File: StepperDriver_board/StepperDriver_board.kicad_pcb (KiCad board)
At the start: 2 copper layers, 50 x 70 mm, 18 parts, among them J1 Conn_01x02, J2 Conn_01x02, J3 Conn_01x02, J4 Conn_01x04_Male, J5 Conn_01x02, J6 Conn_01x04_Male, J7 Conn_01x02, J9 Conn_01x04_Male

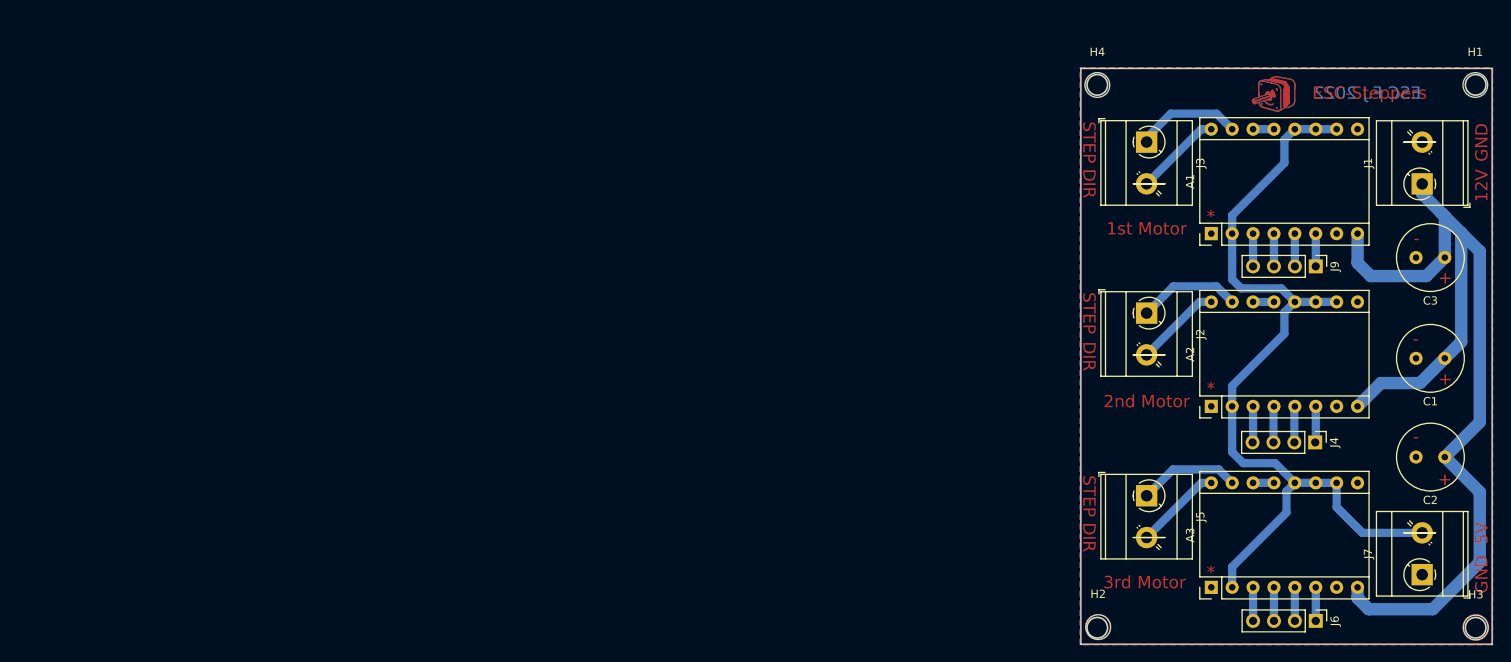
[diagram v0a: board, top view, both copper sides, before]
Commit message: Feat: add assets
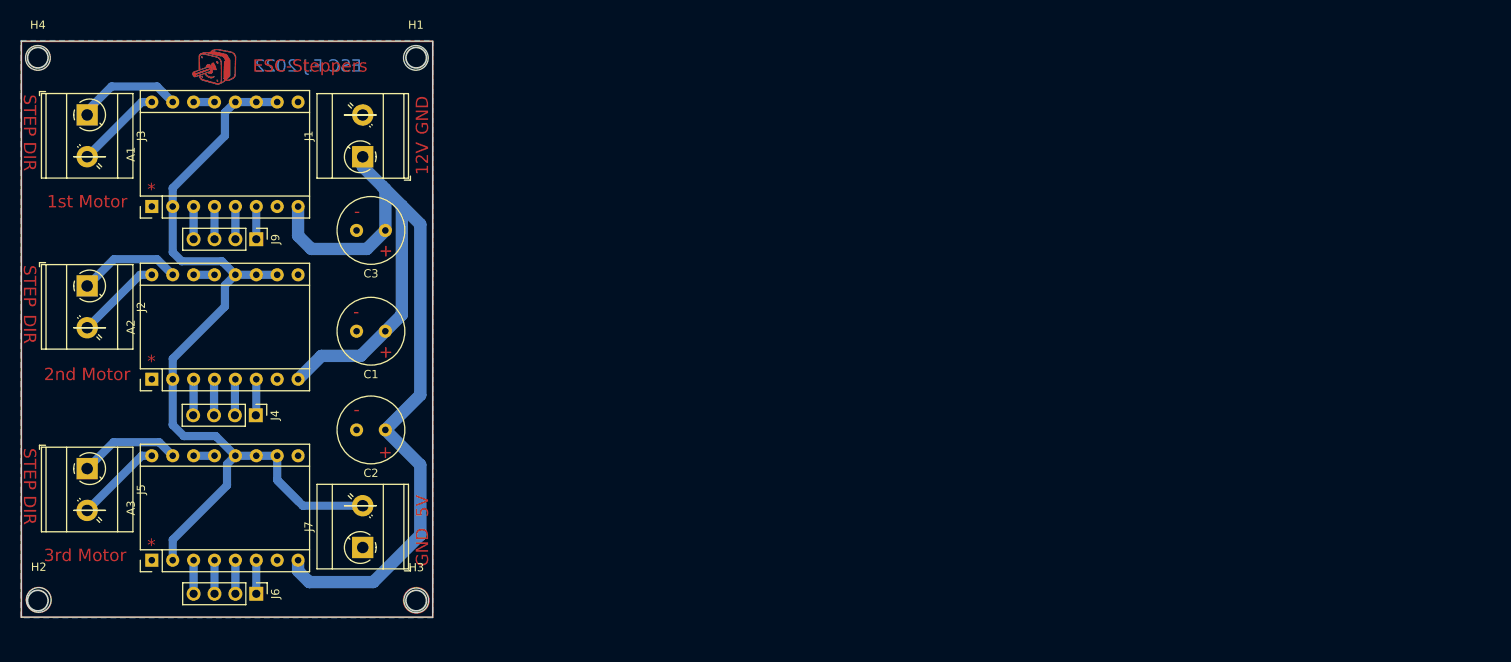
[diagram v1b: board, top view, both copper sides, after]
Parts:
- moved A1 128.8 mm to (-77.0, 39.7)
- moved A2 128.8 mm to (-77.0, 60.7)
- moved A3 128.8 mm to (-77.0, 82.7)
- moved C1 128.8 mm to (-48.6, 54.9)
- moved C2 128.8 mm to (-48.6, 66.9)
- moved C3 128.8 mm to (-48.6, 42.6)
- moved H1 128.8 mm to (-44.9, 21.6)
- moved H2 128.8 mm to (-90.8, 87.5)
- moved H3 128.8 mm to (-44.9, 87.6)
- moved H4 128.8 mm to (-90.8, 21.6)
- moved J1 128.8 mm to (-51.4, 33.7)
- moved J2 128.8 mm to (-84.9, 49.4)
- moved J3 128.8 mm to (-84.9, 28.6)
- moved J4 128.8 mm to (-64.4, 65.1)
- moved J5 128.8 mm to (-84.9, 71.6)
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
